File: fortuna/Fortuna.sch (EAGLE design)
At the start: 36 parts, among them M1 MOTOR20MM, M2 MOTOR20MM, Q1 600mA/40V, Q2 600mA/40V, U2 OPA2343UA, U3 OPA2343UA

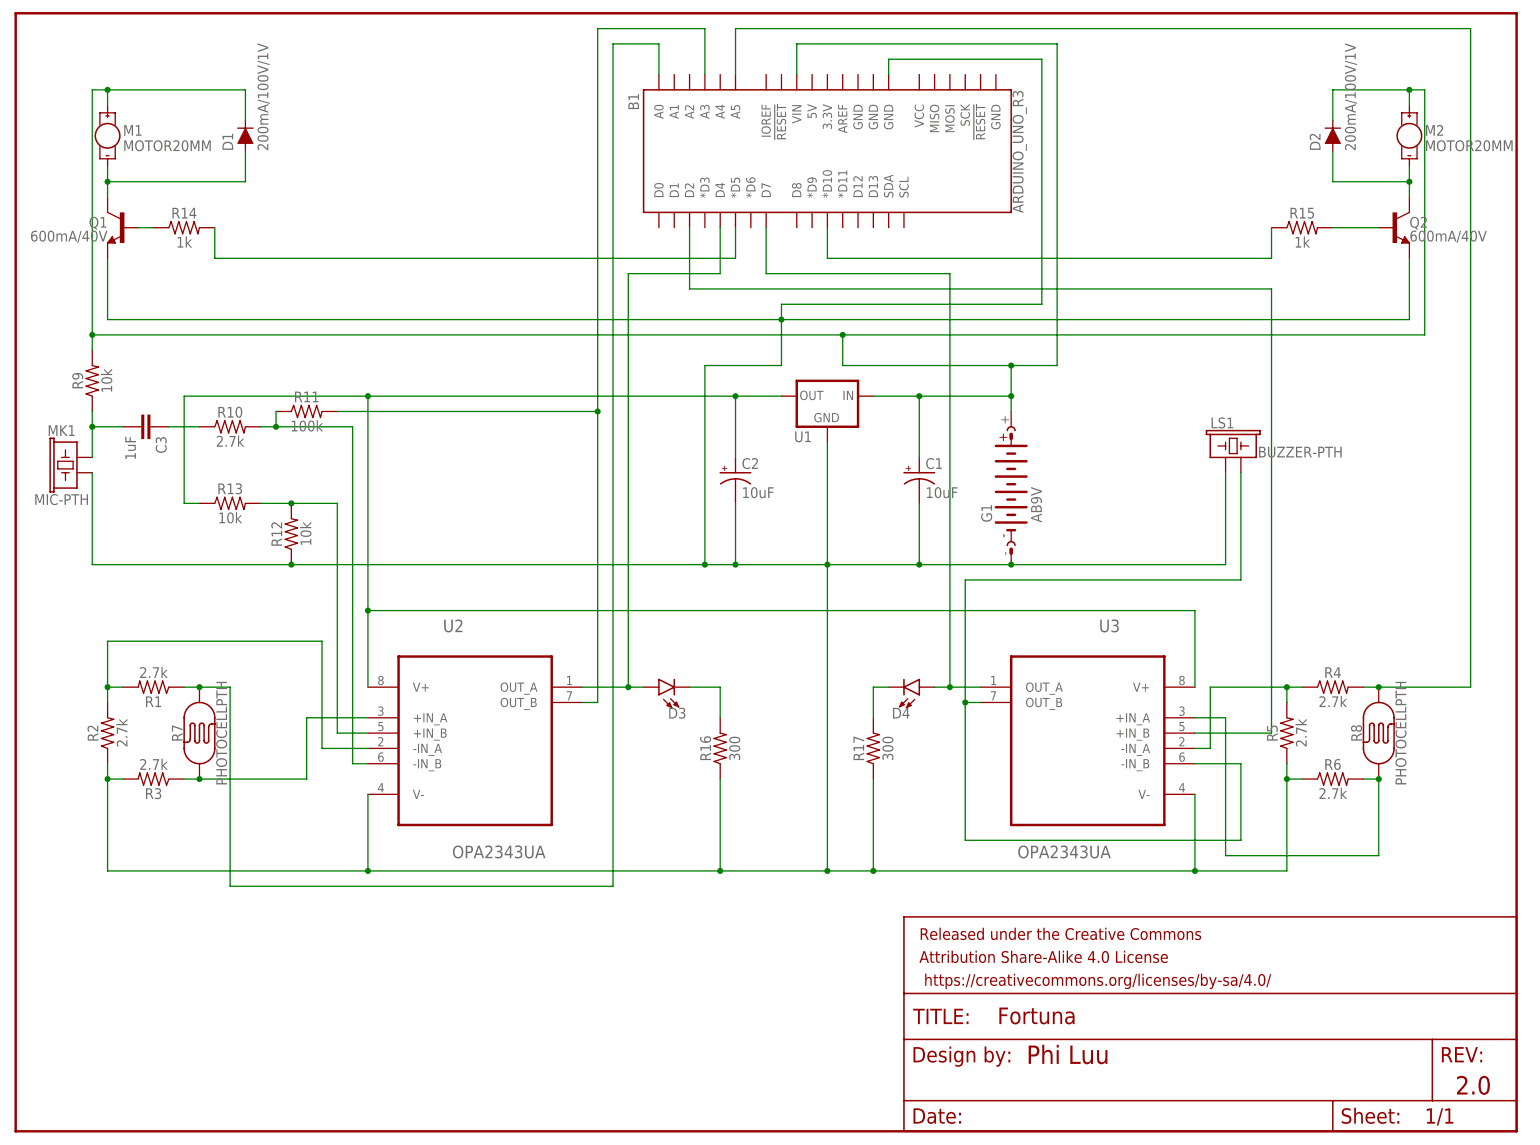
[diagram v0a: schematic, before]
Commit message: Finish fortuna schematic
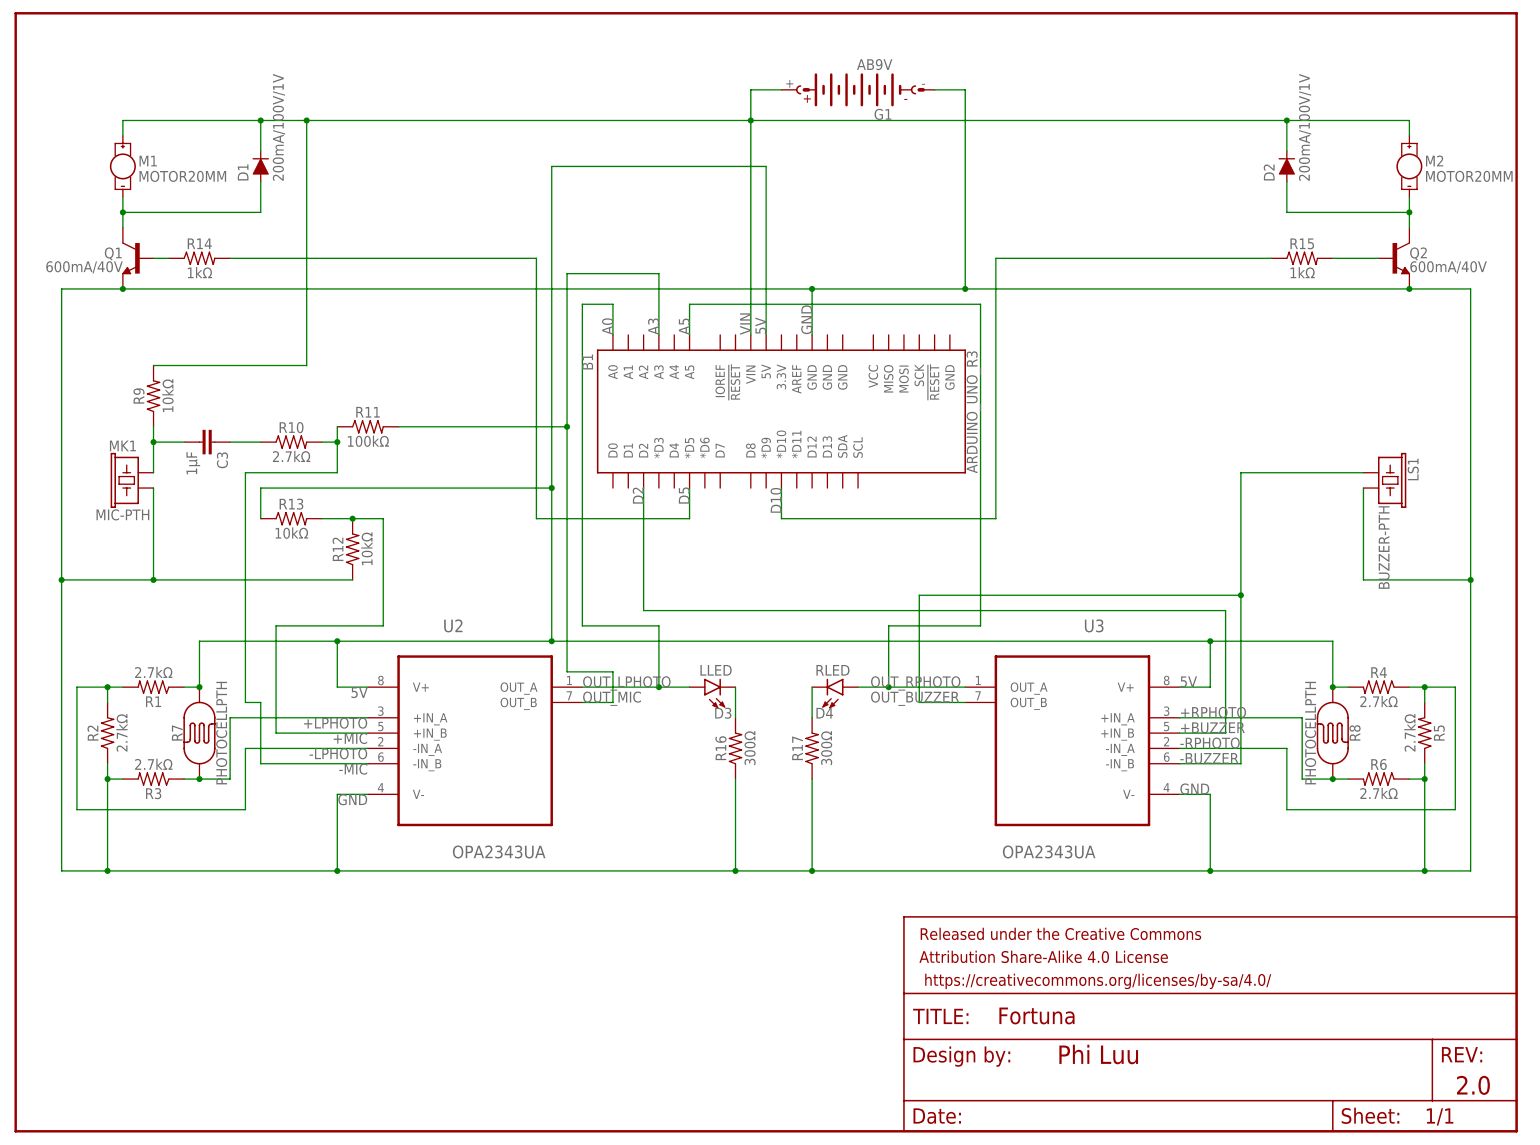
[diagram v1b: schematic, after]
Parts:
- removed C1, C2: 10uF, SparkFun-Capacitors:10UF-POLAR-RADIAL-2.5MM-25V-20%
- removed U1: (no value), SparkFun-IC-Power:V_REG_78XX-TO-220
- C3: value 1uF -> 1μF
- D3: value (none) -> LLED
- D4: value (none) -> RLED
- R1, R10, R2, R3, R4, R5, R6: value 2.7k -> 2.7kΩ
- R11: value 100k -> 100kΩ
- R12, R13, R9: value 10k -> 10kΩ
- R14, R15: value 1k -> 1kΩ
- R16, R17: value 300 -> 300Ω
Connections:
- net N$11 renamed -RPHOTO
- net N$12 renamed D2
- net N$14 renamed -MIC
- net N$15 renamed A3
- net N$25 renamed D5
- net N$26 renamed D10
- net N$4 renamed +MIC
- net N$6 renamed +RPHOTO
- net N$7 renamed -LPHOTO
- net N$9 renamed +LPHOTO
- removed net N$1 (its old number): B1.VIN, C1.+, D1.C, D2.C, G1.+, M1.+, M2.+, R9.2, U1.IN
- removed net N$10 (its old number): B1.A0, R1.1, R7.P$2
- removed net N$16: B1.D4, D3.A, U2.OUT_A
- removed net N$19: B1.D7, D4.A, U3.OUT_A
- removed net N$2 (its old number): B1.GND@0, C1.-, C2.-, G1.-, LS1.1, MK1.2, Q1.E, Q2.E, R12.1, R16.1, R17.1, R2.1, R3.2, R5.1, R6.1, U1.GND, U2.V-, U3.V-
- removed net N$22: B1.A5, R4.2, R8.P$2
- removed net N$3: C2.+, R13.1, U1.OUT, U2.V+, U3.V+
- removed net N$5: LS1.2, U3.-IN_B, U3.OUT_B
- new net 5V: B1.5V, R1.1, R13.1, R4.2, R7.P$2, R8.P$2, U2.V+, U3.V+
- new net A0: B1.A0, D3.A, U2.OUT_A
- new net A5: B1.A5, D4.A, U3.OUT_A
- new net GND: B1.GND@2, G1.-, LS1.2, MK1.2, Q1.E, Q2.E, R12.1, R16.1, R17.1, R2.1, R3.2, R5.1, R6.1, U2.V-, U3.V-
- new net OUT_BUZZER: LS1.1, U3.-IN_B, U3.OUT_B
- new net VIN: B1.VIN, D1.C, D2.C, G1.+, M1.+, M2.+, R9.2
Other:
- note added: "+BUZZER"
- note added: "-BUZZER"
- note added: "OUT_LPHOTO"
- note added: "OUT_MIC"
- note added: "OUT_RPHOTO"
- moved on the sheet: B1, C3, D1, D2, D3, D4, G1, LS1, M1, M2, MK1, Q1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
